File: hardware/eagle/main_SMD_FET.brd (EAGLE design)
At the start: 40 x 31.7 mm, 44 parts, among them IC1 R-78E3.3-1.0, IC2 INA186A1QDCKRQ1, IC3 ESP-12E/F, J4 1727078, Q1 IRFU3710ZPBF, Q2 IRFU3710ZPBF, Q3 IRFU3710ZPBF, Q4 IRFU3710ZPBF

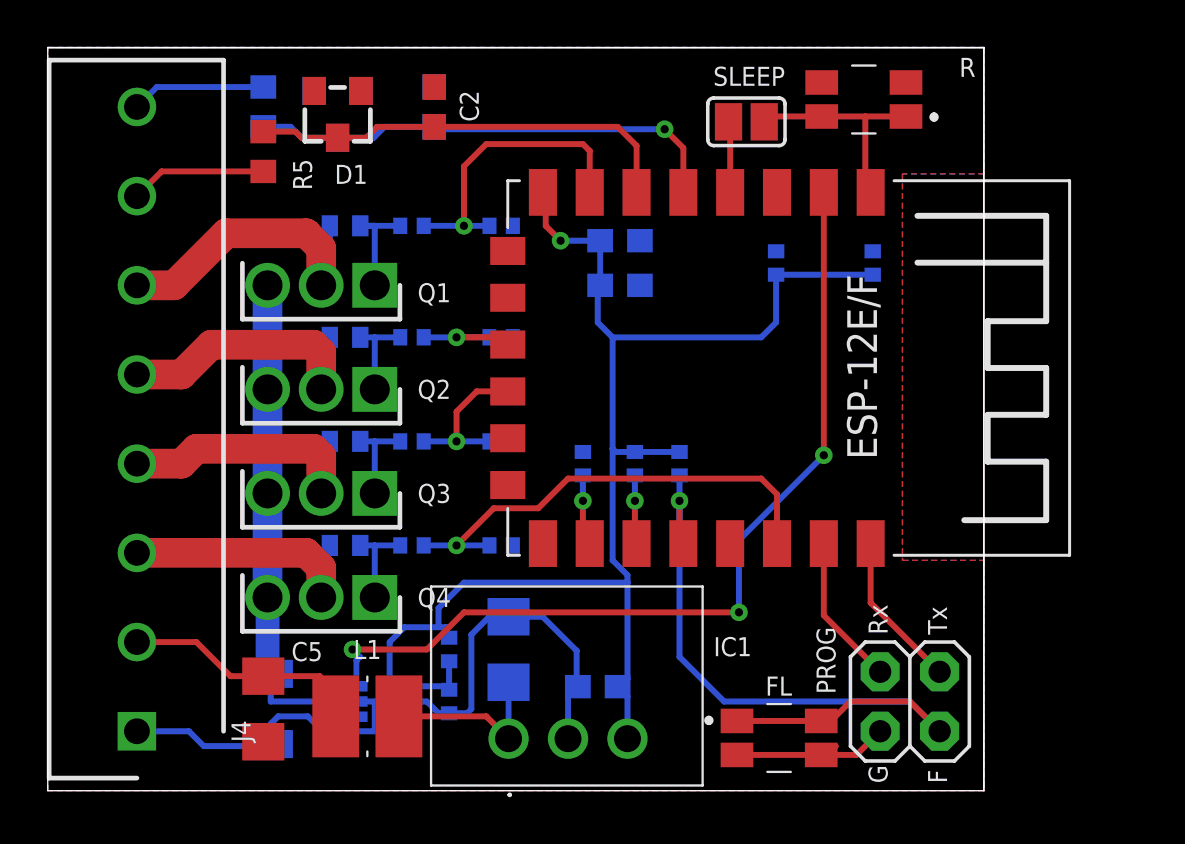
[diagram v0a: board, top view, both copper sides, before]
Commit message: initial
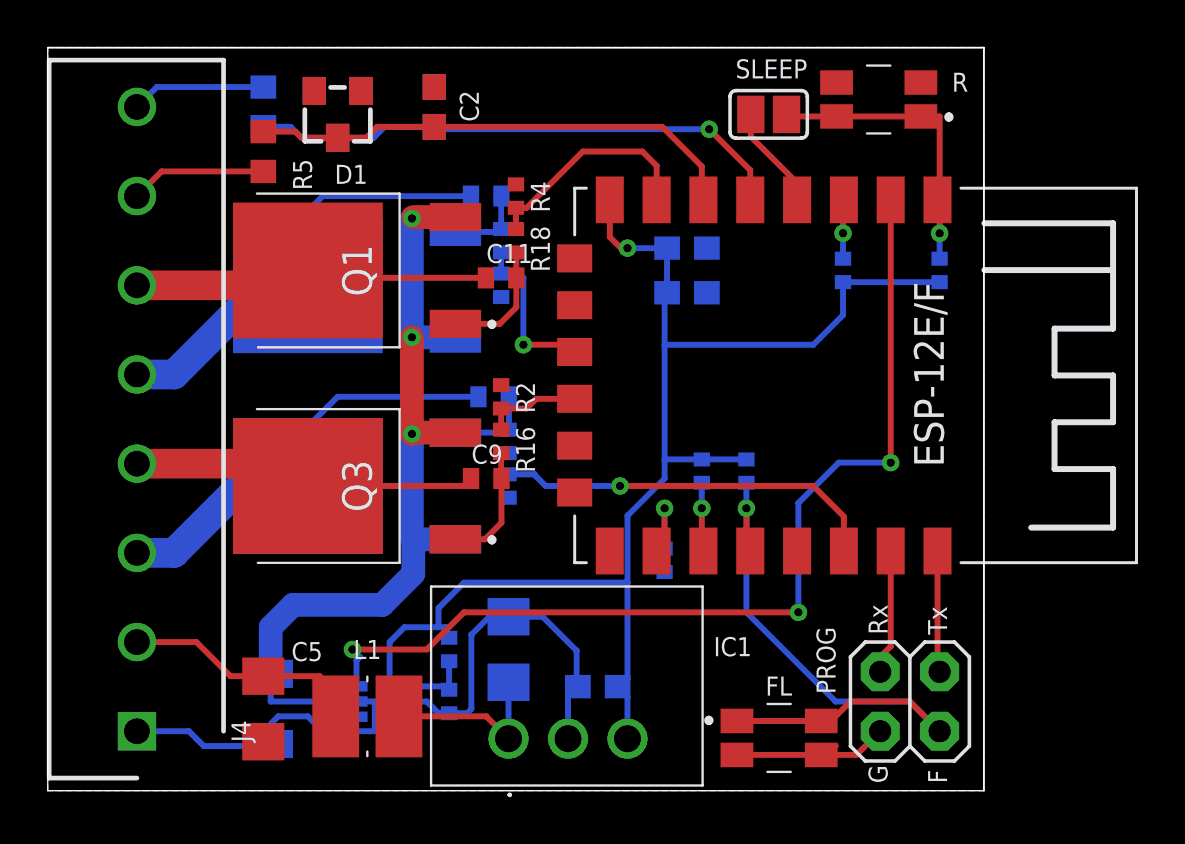
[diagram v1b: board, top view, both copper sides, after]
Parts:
- Q1, Q2, Q3, Q4: value IRFU3710ZPBF -> IPD031N06; device SamacSys_Parts:TO229P239X654X978-3P -> SamacSys_Parts:IPD031N06L3GATMA1
- moved C6 8.98 mm to (19.1, 16.8)
- moved C10 8.53 mm to (18.7, 25.4)
- moved C11 7.03 mm to (19.4, 21.9), flipped to the top, turned to 0 degrees
- moved C9 6.24 mm to (18.7, 13.3), flipped to the top, turned to 0 degrees
- moved R15 6.07 mm to (19.7, 14.9), turned to 90 degrees
- moved R17 5.62 mm to (19.4, 23.5), turned to 90 degrees
- moved Q4 5.55 mm to (11.1, 13.0), flipped to the bottom, turned to 270 degrees
- moved R9 5.41 mm to (26.4, 9.84), turned to 90 degrees
- moved Q2 5.28 mm to (11.1, 21.6), flipped to the bottom, turned to 270 degrees
- moved R18 4.49 mm to (20.0, 23.5), flipped to the top, turned to 270 degrees
- moved R16 3.81 mm to (19.4, 14.9), flipped to the top, turned to 270 degrees
- moved Q1 2.93 mm to (11.1, 22.2), turned to 90 degrees
- moved IC3 2.88 mm to (30.5, 17.8)
- moved R10 2.88 mm to (27.9, 13.7)
- moved R8 2.88 mm to (38.1, 22.2)
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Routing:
- net N$7: track 21.8 -> 37.3 mm, vias 0 -> 3
- net W: track 11.8 -> 18.8 mm
- net G: track 12.5 -> 19.3 mm
- net N$3: track 9.49 -> 14.1 mm, vias 0 -> 1
- net N$13: track 31.6 -> 27.4 mm
- net N$1: track 38.4 -> 42.0 mm
- net W_PIN: track 20.1 -> 16.6 mm
- net R_PIN: track 13.0 -> 9.62 mm, vias 1 -> 0
- net IN_1_PIN: track 18.6 -> 21.3 mm
- net IN_2_PIN: track 20.8 -> 23.4 mm
- net B: track 12.2 -> 14.8 mm
- net N$10: track 0.00 -> 2.53 mm, vias 0 -> 1
- net B_PIN: track 6.63 -> 4.22 mm, vias 1 -> 0
- net G_PIN: track 5.13 -> 7.11 mm
- net R: track 13.3 -> 15.3 mm
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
